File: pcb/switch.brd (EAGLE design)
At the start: 81 x 78.7 mm, 0 parts

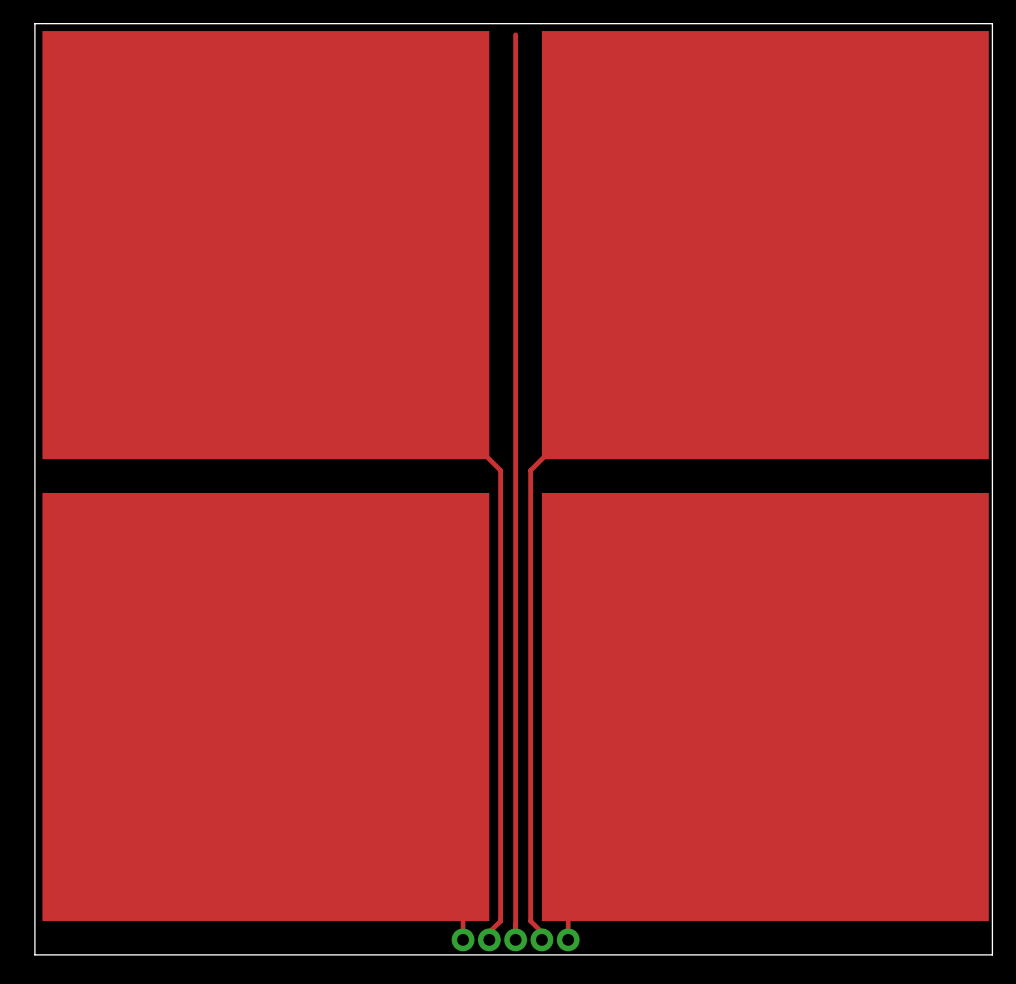
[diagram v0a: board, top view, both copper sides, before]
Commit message: modified
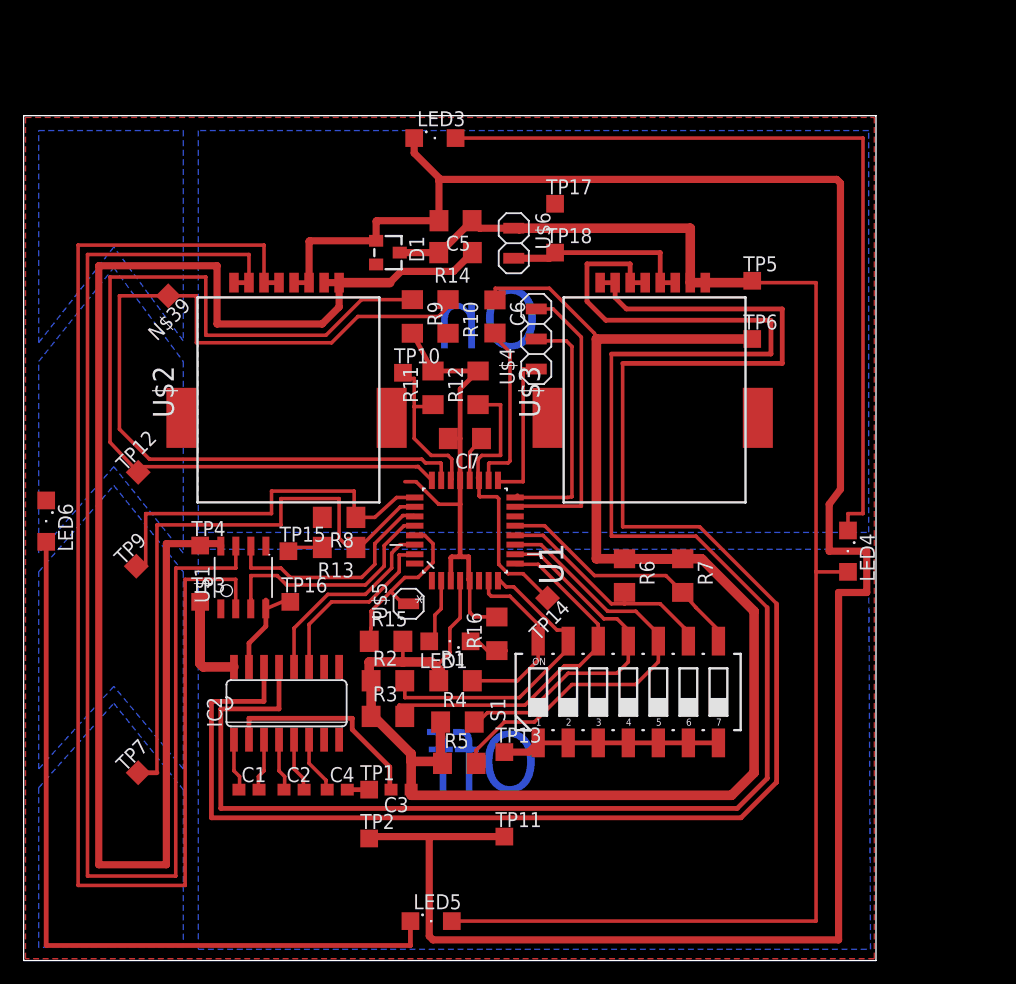
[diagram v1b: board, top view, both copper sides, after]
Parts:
- added C1, C2, C3, C4: (no value), rcl:C0603
- added C5, C6, C7: (no value), rcl:C1206
- added D1: BZX84CSMD, diode:TO236
- added IC2: MAX3232CSE, maxim:SO16
- added LED1, LED3, LED4, LED5, LED6: (no value), led:SML1206
- added N$39, TP1, TP10, TP11, TP12, TP13, TP14, TP15, TP16, TP17, TP18, TP2, TP3, TP4, TP5, TP6, TP7, TP9: TPSQTP15SQ, testpad:TP15SQ
- added R1, R10, R11, R12, R13, R14, R15, R16, R2, R3, R4, R5, R6, R7, R8, R9: (no value), rcl:R1206
- added S1: 219-07, switch-dil:CTS-219-07
- added U$1: P82B715, i2c:P82B715SMD
- added U$2, U$3: RJ45SMD, con-tycoelectronics:RJ45SMD
- added U$4: (no value), pinhead:1X03SMD
- added U$5: PINHD-1X1SMD, pinhead:1X01SMD
- added U$6: PINHD-1X2SMD, pinhead:1X02SMD
- added U1: ATMEGA48-20AU, atmega48:QFP80P900X900X120-32N
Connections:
- new net +12V: IC2.16, R14.1, U$1.8, U$2.P$7, U$2.P$8
- new net GND: C4.2, C5.2, C7.2, D1.A, IC2.15, LED3.C, LED6.C, R10.2, R11.2, R12.2, R13.2, R16.2, R8.2, R9.2, S1.1, S1.2, S1.3, S1.4, S1.5, S1.6, S1.7, TP11.TP, TP13.TP, TP15.TP, TP16.TP, TP17.TP, TP18.TP, TP2.TP, U$1.4, U$2.P$5, U$2.P$6, U$3.P$5, U$3.P$6, U$6.P$2, U1.21, U1.3, U1.5
- new net N$1: U$1.3, U1.28
- new net N$10: IC2.11, U1.31
- new net N$11: IC2.12, U1.30
- new net N$12: U$1.7, U$2.P$1, U$2.P$2
- new net N$13: U$1.2, U$2.P$3, U$2.P$4
- new net N$14: R12.1, TP14.TP, U1.19
- new net N$15: R11.1, TP10.TP, U1.22
- new net N$16: N$39.TP, R10.1, U1.23
- new net N$17: R9.1, TP12.TP, U1.24
- new net N$18: R8.1, TP9.TP, U1.25
- new net N$19: R13.1, TP7.TP, U1.26
- new net N$2: U$1.6, U1.27
- new net N$20: C1.1, IC2.1
- new net N$21: C3.1, C5.1, C6.1, D1.C, LED4.A, LED5.A, R1.1, R14.2, R15.2, R2.1, R3.1, R4.1, R5.1, R6.1, R7.1, TP5.TP, TP6.TP, U$3.P$7, U$3.P$8, U$6.P$1, U1.4, U1.6
- new net N$22: C1.2, IC2.3
- new net N$23: IC2.14, U$3.P$1, U$3.P$2
- new net N$24: IC2.13, U$3.P$3, U$3.P$4
- new net N$25: C2.1, IC2.4
- new net N$26: C2.2, IC2.5
- new net N$27: C3.2, IC2.2
- new net N$28: C4.1, IC2.6
- new net N$29: U$4.P$1, U1.17
- new net N$3: R1.2, S1.14, U1.7
- new net N$30: U$4.P$2, U1.16
- new net N$31: U$4.P$3, U1.15
- new net N$32: R15.1, U$5.P$1, U1.29
- new net N$33: LED1.C, R16.1
- new net N$34: C6.2, U1.18
- new net N$35: LED1.A, U1.2
- new net N$36: C7.1, U1.20
- new net N$37: LED3.A, LED4.C
- new net N$38: LED5.C, LED6.A
- new net N$4: R7.2, S1.8, U1.13
- new net N$5: R6.2, S1.9, U1.12
- new net N$6: R5.2, S1.10, U1.11
- new net N$7: R4.2, S1.11, U1.10
- new net N$8: R3.2, S1.12, U1.9
- new net N$9: R2.2, S1.13, U1.8
- new net VCC: TP3.TP, TP4.TP
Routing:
- net N$4: track 449.6 -> 21.8 mm
- net N$5: track 440.4 -> 19.8 mm
- net N$2: track 384.8 -> 19.3 mm
- net N$8: track 384.8 -> 32.3 mm
- net N$6: track 384.8 -> 37.2 mm
- net N$7: track 377.2 -> 30.5 mm
- net N$3: track 345.4 -> 15.7 mm
- net N$1: track 345.4 -> 20.1 mm
- net N$21: track 0.00 -> 274.5 mm
- net GND: track 0.00 -> 272.9 mm
- net N$24: track 0.00 -> 152.0 mm
- net N$23: track 0.00 -> 146.0 mm
- net +12V: track 0.00 -> 137.6 mm
- net N$12: track 2.99 -> 110.3 mm, vias 1 -> 0
- net N$17: track 0.00 -> 75.0 mm
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- added copper zone on layer 1, net GND
- added copper zone on layer 16, net N$39
- added copper zone on layer 16, net N$40
- added copper zone on layer 16, net N$41
- added copper zone on layer 16, net N$42
- added copper zone on layer 16, net N$43
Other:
- board size 81 x 78.7 mm -> 72.1 x 71.4 mm
- board text added: "Off"
- board text added: "On"

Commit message: sleep mode
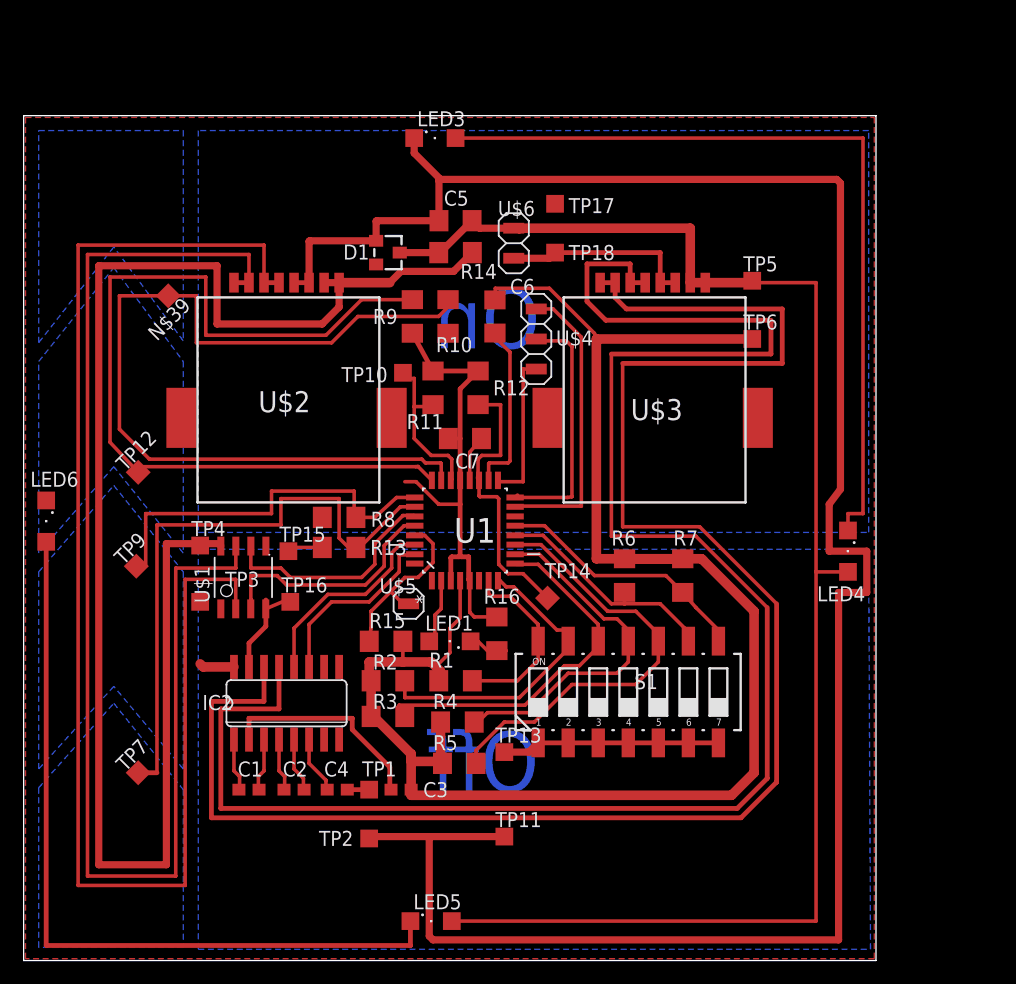
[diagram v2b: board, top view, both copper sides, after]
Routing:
- net +12V: track 137.6 -> 132.7 mm
- net VCC: track 5.24 -> 0.48 mm
